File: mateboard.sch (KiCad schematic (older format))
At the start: 0 parts

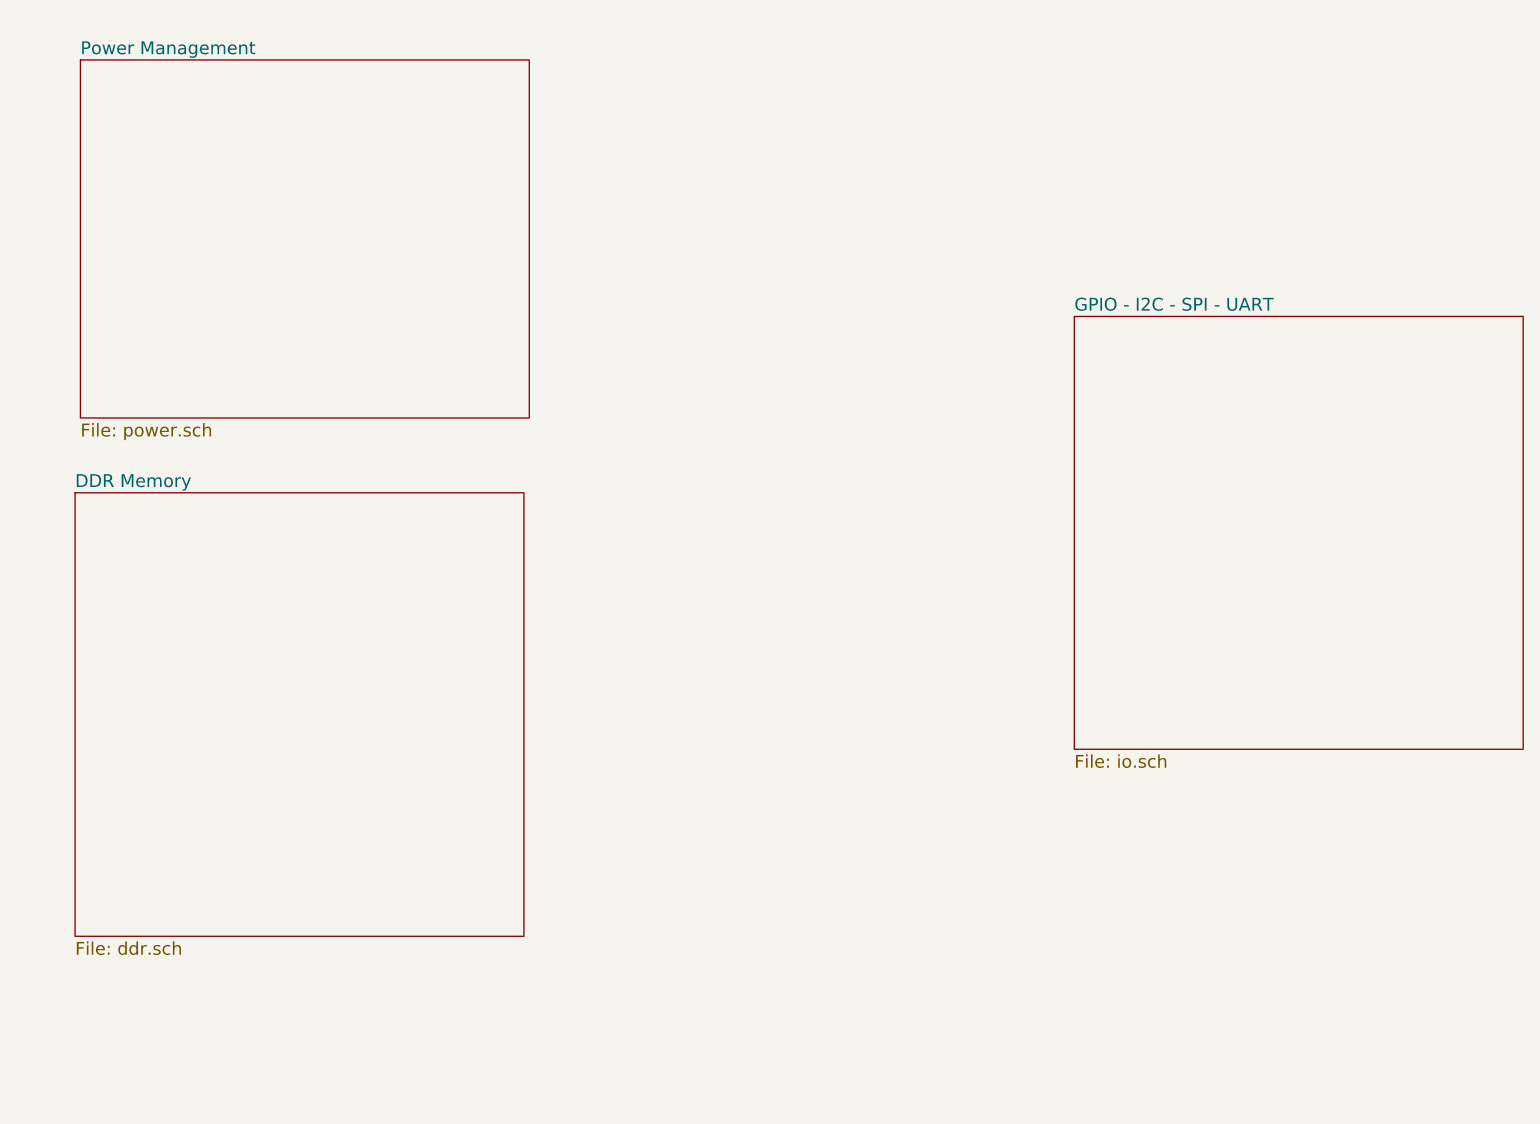
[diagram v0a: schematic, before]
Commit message: power mgmnt done
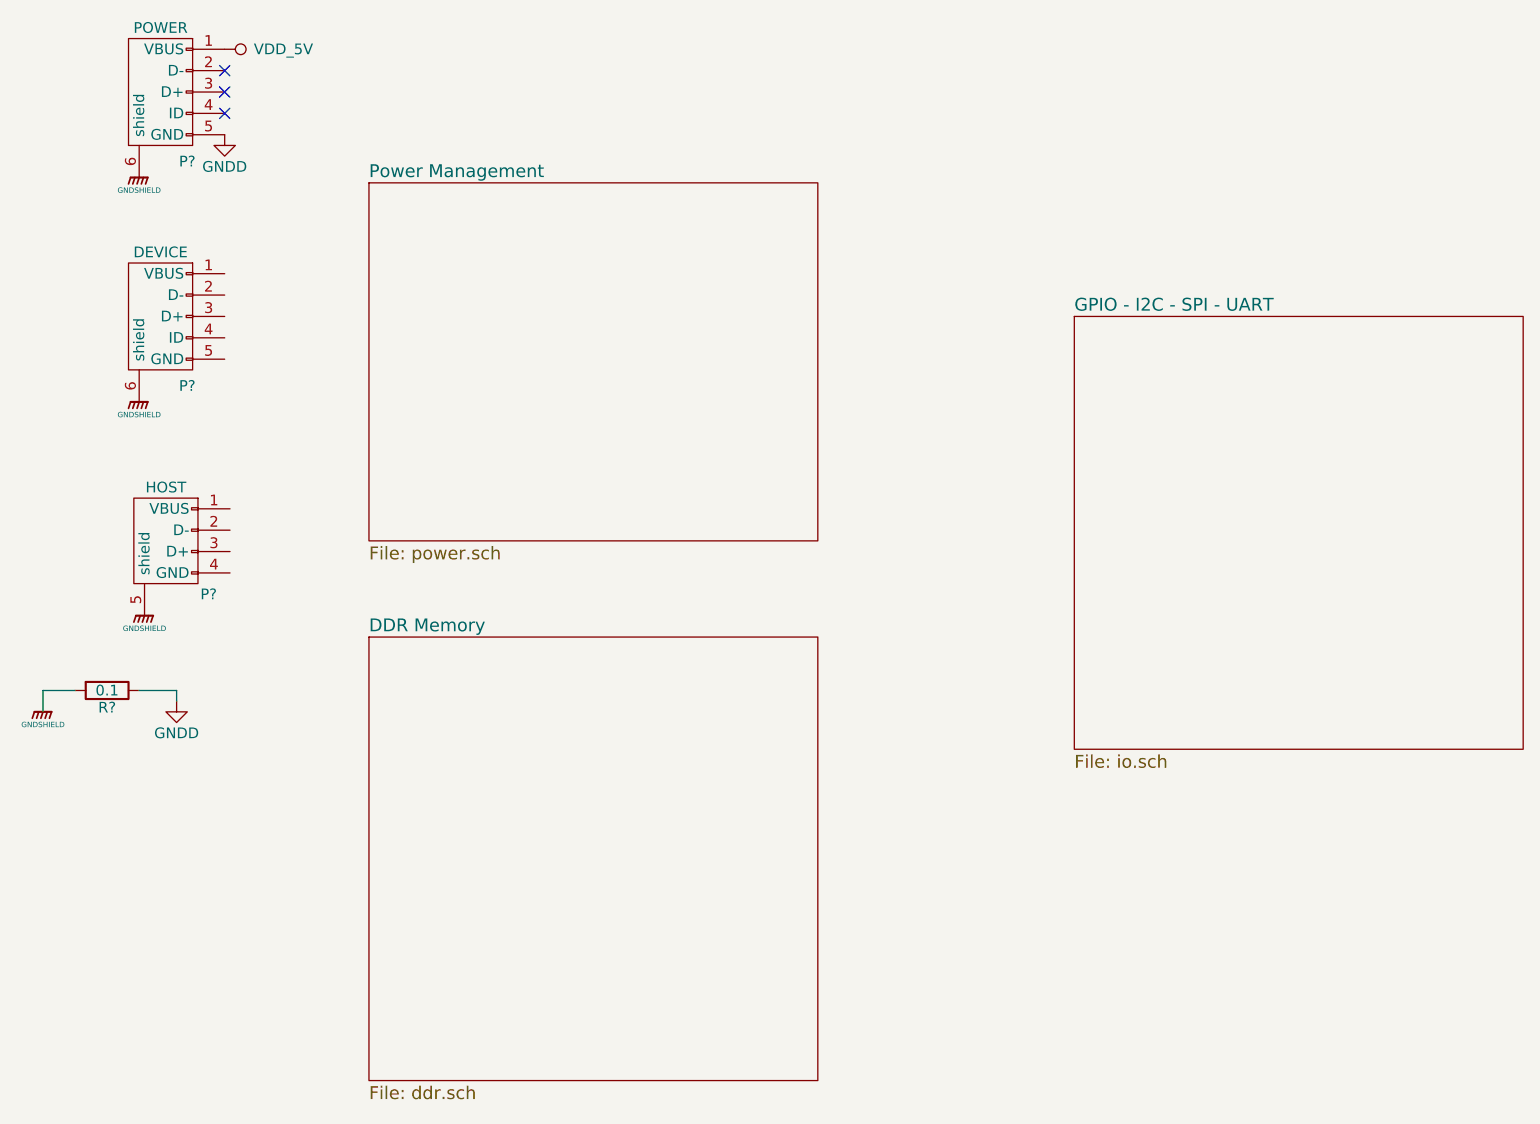
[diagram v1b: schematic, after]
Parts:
- added P?: POWER, symbol USB_OTG
- added P?: HOST, symbol USB_A
- added P?: DEVICE, symbol USB_OTG
- added R?: 0.1, Resistors_SMD:R_0805, symbol R
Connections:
- new net GNDD: P?.5 (GND), R?.1
- new net GNDSHIELD: P?.5 (shield), P?.6 (shield), P?.6 (shield), R?.2
- new net VDD_5V: P?.1 (VBUS)
- no-connect marks 0 -> 3
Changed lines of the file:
@@
 LIBS:tps65217c
 LIBS:pwr
+LIBS:pushbutton
+LIBS:tl5209
+LIBS:tl1963adcqr
 LIBS:mateboard-cache
 EELAYER 25 0
@@
 $EndDescr
 $Sheet
-S 1025 950  2100 1675
+S 2375 1525 2100 1675
 U 589A190D
 F0 "Power Management" 60
@@
 $EndSheet
 $Sheet
-S 1000 2975 2100 2075
+S 2375 3650 2100 2075
 U 589C7F66
 F0 "DDR Memory" 60
@@
 F1 "io.sch" 60
 $EndSheet
+$Comp
+L USB_OTG P?
+U 1 1 589C9196
+P 1400 1100
+F 0 "P?" V 1725 975 50  0000 C CNN
+F 1 "POWER" V 1100 1100 50  0000 C CNN
+F 2 "" V 1350 1000 50  0000 C CNN
+F 3 "" V 1350 1000 50  0000 C CNN
+	1    1400 1100
+	0    -1   1    0
+$EndComp
+$Comp
+L USB_A P?
+U 1 1 589C92E9
+P 1425 3250
+F 0 "P?" V 1625 3050 50  0000 C CNN
+F 1 "HOST" V 1125 3250 50  0000 C CNN
+F 2 "" V 1375 3150 50  0000 C CNN
+F 3 "" V 1375 3150 50  0000 C CNN
+	1    1425 3250
+	0    -1   1    0
+$EndComp
+$Comp
+L USB_OTG P?
+U 1 1 589C94AD
+P 1400 2150
+F 0 "P?" V 1725 2025 50  0000 C CNN
+F 1 "DEVICE" V 1100 2150 50  0000 C CNN
+F 2 "" V 1350 2050 50  0000 C CNN
+F 3 "" V 1350 2050 50  0000 C CNN
+	1    1400 2150
+	0    -1   1    0
+$EndComp
+$Comp
+L GNDD #PWR?
+U 1 1 589C99DB
+P 1700 1300
+F 0 "#PWR?" H 1700 1050 50  0001 C CNN
+F 1 "GNDD" H 1700 1150 50  0000 C CNN
+F 2 "" H 1700 1300 50  0000 C CNN
+F 3 "" H 1700 1300 50  0000 C CNN
+	1    1700 1300
+	1    0    0    -1
+$EndComp
+$Comp
+L VDD_5V #PWR?
+U 1 1 589C99F5
+P 1700 900
+F 0 "#PWR?" H 1700 750 50  0001 C CNN
+F 1 "VDD_5V" V 1700 1175 50  0000 C CNN
+F 2 "" H 1700 900 50  0000 C CNN
+F 3 "" H 1700 900 50  0000 C CNN
+	1    1700 900
+	0    1    1    0
+$EndComp
+NoConn ~ 1700 1000
+NoConn ~ 1700 1100
+NoConn ~ 1700 1200
+$Comp
+L GNDSHIELD #PWR?
+U 1 1 589C9AC7
+P 1300 1500
+F 0 "#PWR?" H 1300 1550 40  0001 C CNN
+F 1 "GNDSHIELD" H 1300 1440 25  0000 C CNN
+F 2 "" H 1300 1500 60  0001 C CNN
+F 3 "" H 1300 1500 60  0001 C CNN
+	1    1300 1500
+	1    0    0    -1
+$EndComp
+$Comp
+L GNDSHIELD #PWR?
+U 1 1 589C9BDB
+P 1325 3550
+F 0 "#PWR?" H 1325 3600 40  0001 C CNN
+F 1 "GNDSHIELD" H 1325 3490 25  0000 C CNN
+F 2 "" H 1325 3550 60  0001 C CNN
+F 3 "" H 1325 3550 60  0001 C CNN
+	1    1325 3550
+	1    0    0    -1
+$EndComp
+$Comp
+L GNDSHIELD #PWR?
+U 1 1 589C9C79
+P 1300 2550
+F 0 "#PWR?" H 1300 2600 40  0001 C CNN
+F 1 "GNDSHIELD" H 1300 2490 25  0000 C CNN
+F 2 "" H 1300 2550 60  0001 C CNN
+F 3 "" H 1300 2550 60  0001 C CNN
+	1    1300 2550
+	1    0    0    -1
+$EndComp
+$Comp
+L GNDSHIELD #PWR?
+U 1 1 589C9CB7
+P 850 4000
+F 0 "#PWR?" H 850 4050 40  0001 C CNN
+F 1 "GNDSHIELD" H 850 3940 25  0000 C CNN
+F 2 "" H 850 4000 60  0001 C CNN
+F 3 "" H 850 4000 60  0001 C CNN
+	1    850  4000
+	1    0    0    -1
+$EndComp
+$Comp
+L GNDD #PWR?
+U 1 1 589C9CCE
+P 1475 3950
+F 0 "#PWR?" H 1475 3700 50  0001 C CNN
+F 1 "GNDD" H 1475 3800 50  0000 C CNN
+F 2 "" H 1475 3950 50  0000 C CNN
+F 3 "" H 1475 3950 50  0000 C CNN
+	1    1475 3950
+	1    0    0    -1
+$EndComp
+$Comp
+L R R?
+U 1 1 589C9CED
+P 1150 3900
+F 0 "R?" V 1230 3900 50  0000 C CNN
+F 1 "0.1" V 1150 3900 50  0000 C CNN
+F 2 "Resistors_SMD:R_0805" V 1080 3900 50  0001 C CNN
+F 3 "" H 1150 3900 50  0000 C CNN
+	1    1150 3900
+	0    1    1    0
+$EndComp
+Wire Wire Line
+	1000 3900 850  3900
+Wire Wire Line
+	850  3900 850  4000
+Wire Wire Line
+	1300 3900 1475 3900
+Wire Wire Line
+	1475 3900 1475 3950
 $EndSCHEMATC
